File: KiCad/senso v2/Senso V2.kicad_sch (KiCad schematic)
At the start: 17 parts

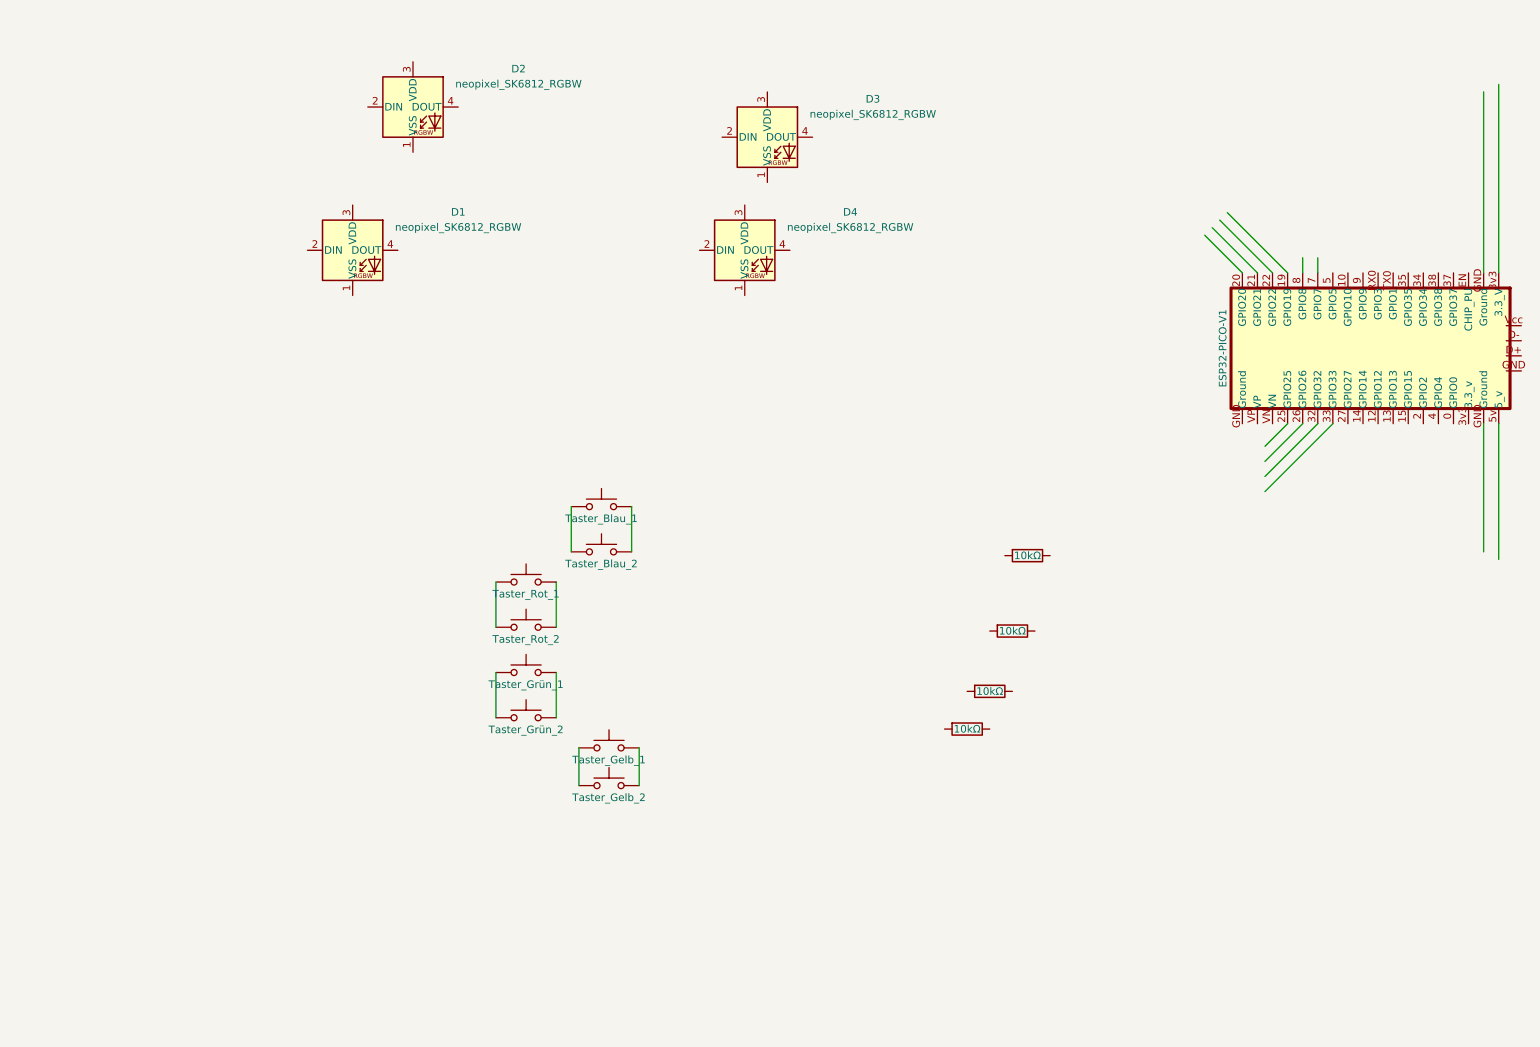
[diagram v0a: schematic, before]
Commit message: update KiCad
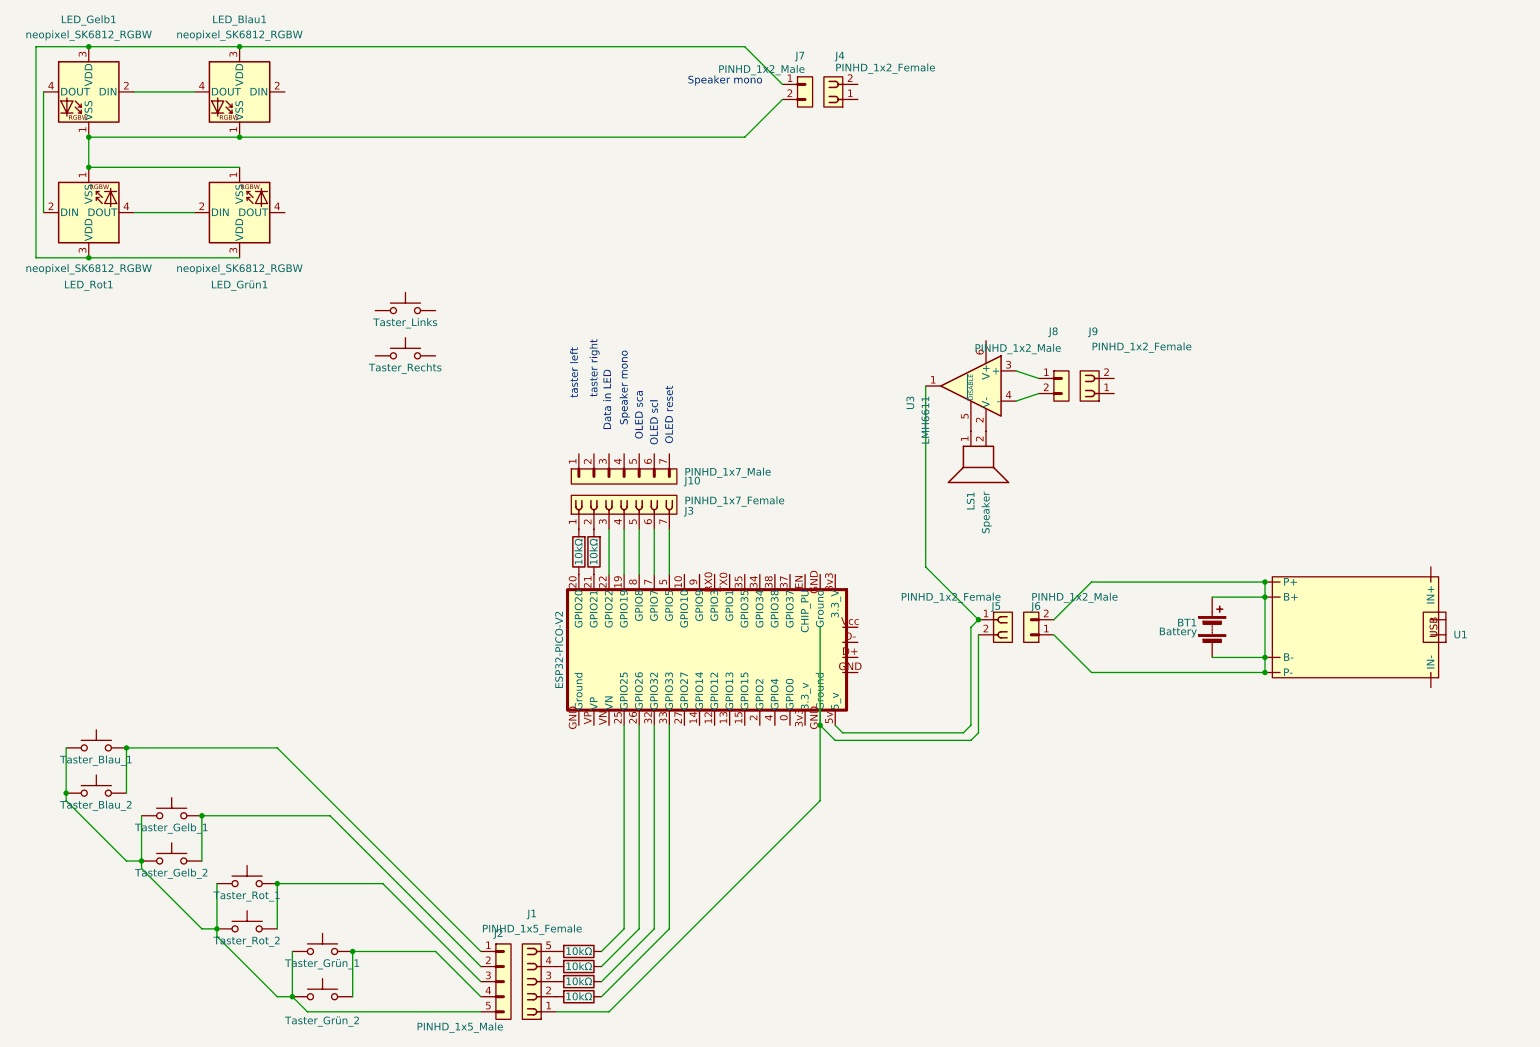
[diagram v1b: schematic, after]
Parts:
- removed ESP32-PICO-V1: ESP32-PICO-V3, senso:ESP32-PICO-V3, symbol senso:ESP32-PICO-V3
- added BT1: Battery, symbol Device:Battery
- added ESP32-PICO-V2: ESP32-PICO-V3, senso:ESP32-PICO-V3, symbol senso_lib:ESP32-PICO-V3
- added J1: PINHD_1x5_Female, Connector_PinSocket_2.54mm:PinSocket_1x05_P2.54mm_Vertical, symbol PCM_SL_Pin_Headers:PINHD_1x5_Female
- added J10: PINHD_1x7_Male, Connector_PinHeader_2.54mm:PinHeader_1x07_P2.54mm_Vertical, symbol PCM_SL_Pin_Headers:PINHD_1x7_Male
- added J2: PINHD_1x5_Male, Connector_PinHeader_2.54mm:PinHeader_1x05_P2.54mm_Vertical, symbol PCM_SL_Pin_Headers:PINHD_1x5_Male
- added J3: PINHD_1x7_Female, Connector_PinSocket_2.54mm:PinSocket_1x07_P2.54mm_Vertical, symbol PCM_SL_Pin_Headers:PINHD_1x7_Female
- added J4, J5, J9: PINHD_1x2_Female, Connector_PinSocket_2.54mm:PinSocket_1x02_P2.54mm_Vertical, symbol PCM_SL_Pin_Headers:PINHD_1x2_Female
- added J6, J7, J8: PINHD_1x2_Male, Connector_PinHeader_2.54mm:PinHeader_1x02_P2.54mm_Vertical, symbol PCM_SL_Pin_Headers:PINHD_1x2_Male
- added LS1: Speaker, symbol Device:Speaker
- added R1, R2: 10kΩ, symbol Device:R
- added Taster_Links, Taster_Rechts: SW_Omron_B3FS, symbol Switch:SW_Omron_B3FS
- added U1: ~, symbol senso_lib:charge_controller
- added U3: LMH6611, Package_TO_SOT_SMD:TSOT-23-6, symbol Amplifier_Operational:LMH6611
- renumbered D1 to LED_Blau1, D4 to LED_Gelb1, D3 to LED_Grün1, D2 to LED_Rot1
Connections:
- net at LED_Blau1.1 (VSS): now also LED_Gelb1.1 (VSS), LED_Grün1.1 (VSS), LED_Rot1.1 (VSS), J7.2
- net at LED_Blau1.3 (VDD): now also LED_Gelb1.3 (VDD), LED_Grün1.3 (VDD), LED_Rot1.3 (VDD), J7.1
- net at LED_Blau1.4 (DOUT): now also LED_Gelb1.2 (DIN)
- net at Taster_Rot_1.1, Taster_Rot_2.1: now also Taster_Blau_1.1, Taster_Blau_2.1, Taster_Gelb_1.1, Taster_Gelb_2.1, Taster_Grün_1.1, Taster_Grün_2.1, J2.5
- net at Taster_Rot_1.2, Taster_Rot_2.2: now also J2.3
- net at Taster_Grün_1.2, Taster_Grün_2.2: now also J2.4
- net at R5.1: now also ESP32-PICO-V2.25 (GPIO25)
- net at R5.2: now also J1.5
- net at R8.1: now also ESP32-PICO-V2.33 (GPIO33)
- net at R8.2: now also J1.2
- net at Taster_Gelb_1.2, Taster_Gelb_2.2: now also J2.2
- net at Taster_Blau_1.2, Taster_Blau_2.2: now also J2.1
- net at LED_Rot1.2 (DIN): now also LED_Gelb1.4 (DOUT)
- net at LED_Rot1.4 (DOUT): now also LED_Grün1.2 (DIN)
- net at R7.1: now also ESP32-PICO-V2.32 (GPIO32)
- net at R7.2: now also J1.3
- net at R6.1: now also ESP32-PICO-V2.26 (GPIO26)
- net at R6.2: now also J1.4
- new net: ESP32-PICO-V2.5v (5_v), J5.1, U3.1
- new net: ESP32-PICO-V2.GND (Ground), J1.1, J5.2
- new net: LS1.1, U3.5 (~{DISABLE})
- new net: LS1.2, U3.2 (V-)
- new net: J8.1, U3.3 (+)
- new net: J8.2, U3.4 (-)
- new net: J3.1, R2.2
- new net: J3.2, R1.2
- new net: ESP32-PICO-V2.22 (GPIO22), J3.3
- new net: ESP32-PICO-V2.19 (GPIO19), J3.4
- new net: ESP32-PICO-V2.8 (GPIO8), J3.5
- new net: ESP32-PICO-V2.7 (GPIO7), J3.6
- new net: ESP32-PICO-V2.5 (GPIO5), J3.7
- new net: ESP32-PICO-V2.20 (GPIO20), R2.1
- new net: BT1.1 (+), BT1.2 (-), J6.1, J6.2, U1. (IN+)
- new net: ESP32-PICO-V2.21 (GPIO21), R1.1
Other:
- note added: "Data in LED"
- note added: "OLED reset"
- note added: "OLED sca"
- note added: "OLED scl"
- note added: "Speaker mono"
- note added: "taster left"
- note added: "taster right"
- moved on the sheet: LED_Blau1, LED_Gelb1, LED_Grün1, LED_Rot1, Taster_Blau_1, Taster_Blau_2, Taster_Gelb_1, Taster_Gelb_2, Taster_Grün_1, Taster_Grün_2, Taster_Rot_1, Taster_Rot_2
